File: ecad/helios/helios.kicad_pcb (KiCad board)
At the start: 2 copper layers, 107 parts, among them J1 JST SH, J10 JST PH, J11 Phoenix MCV_1,5, J12 Phoenix MCV_1,5, J13 Phoenix MCV_1,5, J15 Phoenix MCV_1,5, J16 Phoenix MCV_1,5, J17 Phoenix MCV_1,5, J2 JST SH, J3 Jack-DC OD 5.5 IN 2.1, J4 JST XH, J5 JST XH, J6 JST XH, J7 JST XH, J8 .100 Header, J9 JST PH, Q1 RE1C002UN, Q2 RE1C002UN, Q3 DMG2305UX, U1 W25Q16JVUXIQ, U10 LTV-827S, U12 LTV-827S, U2 RP2040, U3 LMR36501P3RPE, U4 THVD8010, U5 THVD8010, U6 THVD8010, U7 THVD8010, U8 TCAN3414, U9 74LVC1G17, Y1 ABM8-272-T3

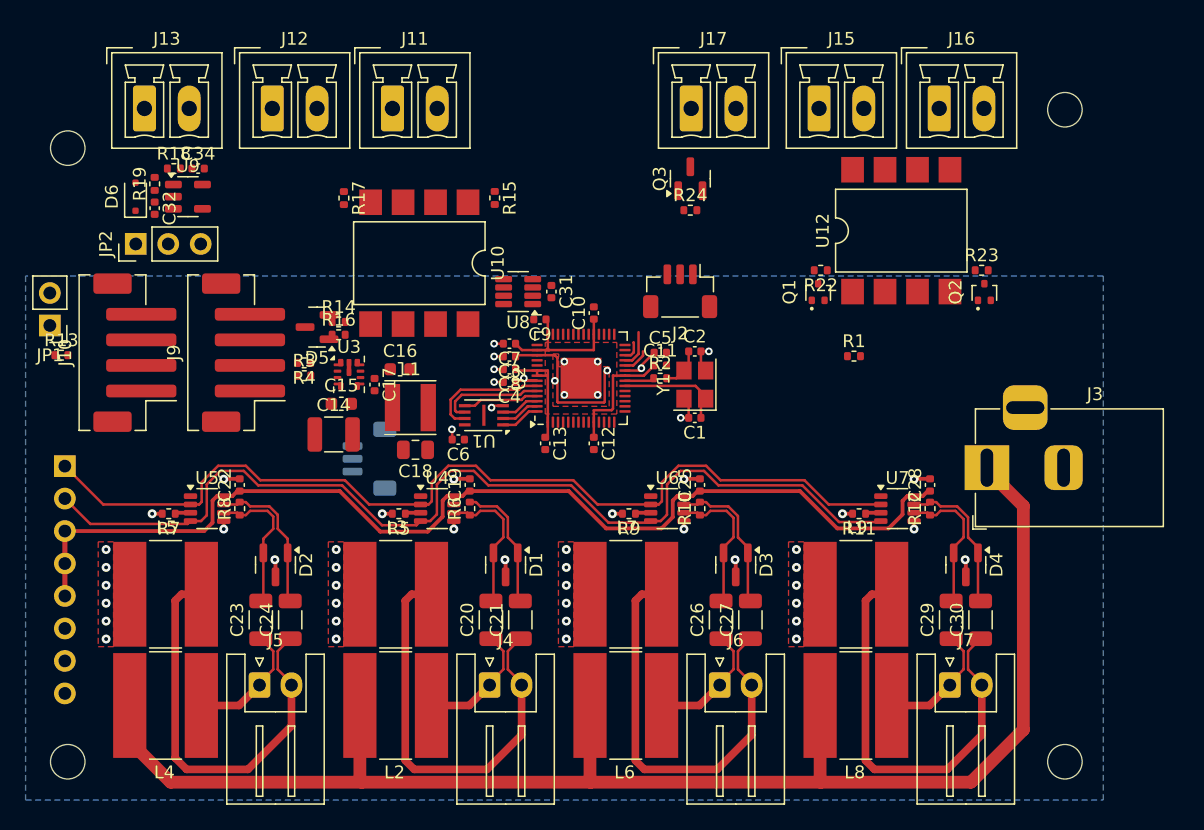
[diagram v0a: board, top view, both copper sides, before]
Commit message: Layouts Helios MkII
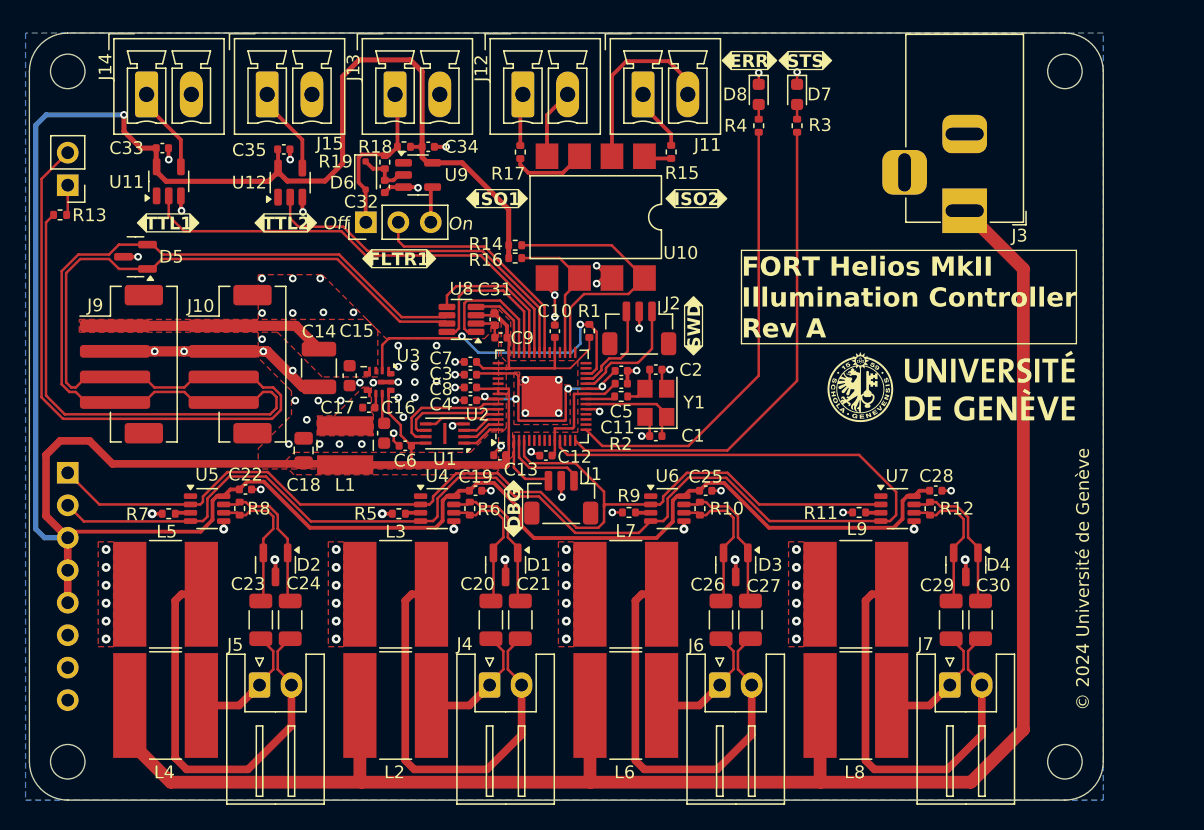
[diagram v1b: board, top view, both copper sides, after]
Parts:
- removed J16, J17: Phoenix MCV_1,5, Connector_Phoenix_MC:PhoenixContact_MCV_1,5_2-G-3.5_1x02_P3.50mm_Vertical
- removed Q1, Q2: RE1C002UN, Package_TO_SOT_SMD:SOT-416
- removed Q3: DMG2305UX, Package_TO_SOT_SMD:SOT-23
- removed R22, R23: 220, Resistor_SMD:R_0402_1005Metric
- removed R24: 15k, Resistor_SMD:R_0402_1005Metric
- added C33: 100n, Capacitor_SMD:C_0402_1005Metric, F.Cu at (136.4, 90.0)
- added C35: 100n, Capacitor_SMD:C_0402_1005Metric, F.Cu at (145.9, 90.1)
- added D7: GREEN, LED_SMD:LED_0603_1608Metric, F.Cu at (186.1, 85.8)
- added D8: YELLOW, LED_SMD:LED_0603_1608Metric, F.Cu at (183.1, 85.8)
- added J14: Phoenix MCV_1,5, Connector_Phoenix_MC:PhoenixContact_MCV_1,5_2-G-3.5_1x02_P3.50mm_Vertical, F.Cu at (135.2, 85.8)
- added U11: 74LVC1G17, Package_TO_SOT_SMD:SOT-23-5, F.Cu at (136.9, 92.6)
- J1: moved to F.Cu
- L1: value 47u -> 22u; footprint Inductor_SMD:L_Taiyo-Yuden_NR-40xx -> fort:L_Wuerth_WE-LQS_4025
- R3: value 7.5k -> 60
- R4: value 10k -> 240
- U12: value LTV-827S -> 74LVC1G17; footprint Package_DIP:SMDIP-8_W9.53mm -> Package_TO_SOT_SMD:SOT-23-5
- U3: value LMR36501P3RPE -> LMR36502P3RPE
- moved U12 47.9 mm to (146.4, 92.7)
- moved R3 43.2 mm to (186.1, 88.2), turned to -90 degrees
- moved J15 43.2 mm to (144.6, 85.8)
- moved R4 40.1 mm to (183.1, 88.2), turned to -90 degrees
- moved R1 20.8 mm to (169.8, 104.3), turned to 90 degrees
- moved J3 20.2 mm to (199.2, 94.9), turned to -90 degrees
- moved J11 19.6 mm to (174.0, 85.8)
- moved J12 19.6 mm to (164.6, 85.8)
- moved J13 19.6 mm to (154.6, 85.8)
- moved C32 18.1 mm to (153.8, 93.0)
- moved C34 18.1 mm to (157.2, 89.9)
- moved JP2 18.1 mm to (152.3, 95.8)
- moved R18 18.1 mm to (155.3, 89.9)
- moved R19 18.1 mm to (153.8, 91.1)
- moved U9 18.1 mm to (156.4, 92.1)
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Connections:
- J15 pad 2: Net-(J15-Pin_2) -> GND
- JP1 pad 2: /CAN- -> /CAN+
- R13 pad 2: /CAN+ -> /CAN-
- R3 pad 1: +12V -> Net-(D7-A)
- R3 pad 2: /RG_EN -> /LED_G
- R4 pad 1: /RG_EN -> Net-(D8-A)
- R4 pad 2: GND -> /LED_Y
- U12 pad 1: Net-(R22-Pad1) -> unconnected-(U12-NC-Pad1)
- U12 pad 2: Net-(Q1-D) -> /OUT_2
- U12 pad 3: Net-(R23-Pad1) -> GND
- U12 pad 4: Net-(Q2-D) -> Net-(J15-Pin_1)
- U12 pad 5: Net-(J16-Pin_2) -> +3V3
- U2 pad 11: /~{OUT_HS1} -> /TX
- U2 pad 12: /~{OUT_HS2} -> unconnected-(U2-GPIO9-Pad12)
- U2 pad 14: unconnected-(U2-GPIO11-Pad14) -> /LED_G
- U2 pad 15: /CAN_TX -> /LED_Y
- U2 pad 16: /CAN_RX -> unconnected-(U2-GPIO13-Pad16)
- U2 pad 17: /CAN_SHUTDOWN -> unconnected-(U2-GPIO14-Pad17)
- U2 pad 18: /CAN_STDBY -> unconnected-(U2-GPIO15-Pad18)
- U2 pad 30: unconnected-(U2-GPIO19-Pad30) -> /IN_ISO1
- U2 pad 31: unconnected-(U2-GPIO20-Pad31) -> /IN_ISO2
- U2 pad 34: /PWM_FAN -> unconnected-(U2-GPIO22-Pad34)
- U2 pad 35: /PWM_HEAT -> /IN_OC1
- U2 pad 36: unconnected-(U2-GPIO24-Pad36) -> /OUT_2
- U2 pad 37: unconnected-(U2-GPIO25-Pad37) -> /OUT_1
- U2 pad 38: unconnected-(U2-GPIO26_ADC0-Pad38) -> /CAN_SHUTDOWN
- U2 pad 39: unconnected-(U2-GPIO27_ADC1-Pad39) -> /CAN_STDBY
- U2 pad 4: unconnected-(U2-GPIO2-Pad4) -> /DE
- U2 pad 40: unconnected-(U2-GPIO28_ADC2-Pad40) -> /CAN_TX
- U2 pad 41: unconnected-(U2-GPIO29_ADC3-Pad41) -> /CAN_RX
- U2 pad 7: /DE -> unconnected-(U2-GPIO5-Pad7)
- U2 pad 8: /TX -> unconnected-(U2-GPIO6-Pad8)
- U3 pad 3: /RG_EN -> +12V
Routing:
- net +3V3: track 115.2 -> 279.8 mm, vias 0 -> 1
- net /CAN+: track 0.00 -> 101.0 mm
- net /CAN-: track 0.00 -> 94.9 mm
- net GND: track 25.3 -> 68.1 mm, vias 52 -> 103
- net /LED_G: track 0.00 -> 39.4 mm
- net /OUT_1: track 0.00 -> 36.6 mm
- net /LED_Y: track 0.00 -> 35.4 mm
- net /TX: track 79.1 -> 107.4 mm
- net /OUT_2: track 0.00 -> 27.6 mm
- net /RUN: track 1.57 -> 25.5 mm, vias 0 -> 2
- net +48V: track 115.3 -> 136.4 mm
- net /IN_ISO1: track 0.00 -> 20.9 mm
- net /IN_OC1: track 0.00 -> 18.6 mm
- net +12V: track 0.00 -> 16.7 mm
- net Net-(J11-Pin_2): track 0.00 -> 14.4 mm
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- added copper zone on F.Cu, net +12V
- added copper zone on F.Cu, net /RG_SW
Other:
- board outline added: 84 x 60 mm
- board text added: "DBG"
- board text added: "ERR"
- board text added: "FLTR1"
- board text added: "FORT Helios MkII Illumination Controller Rev A"
- board text added: "ISO1"
- board text added: "ISO2"
- board text added: "Off"
- board text added: "On"
- board text added: "STS"
- board text added: "SWD"
- board text added: "TTL1"
- board text added: "TTL2"
- board text added: "© 2024 Université de Genève"
